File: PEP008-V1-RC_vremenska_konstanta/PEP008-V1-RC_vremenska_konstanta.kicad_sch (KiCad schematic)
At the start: 23 parts, among them J1 Screw_Terminal_01x02

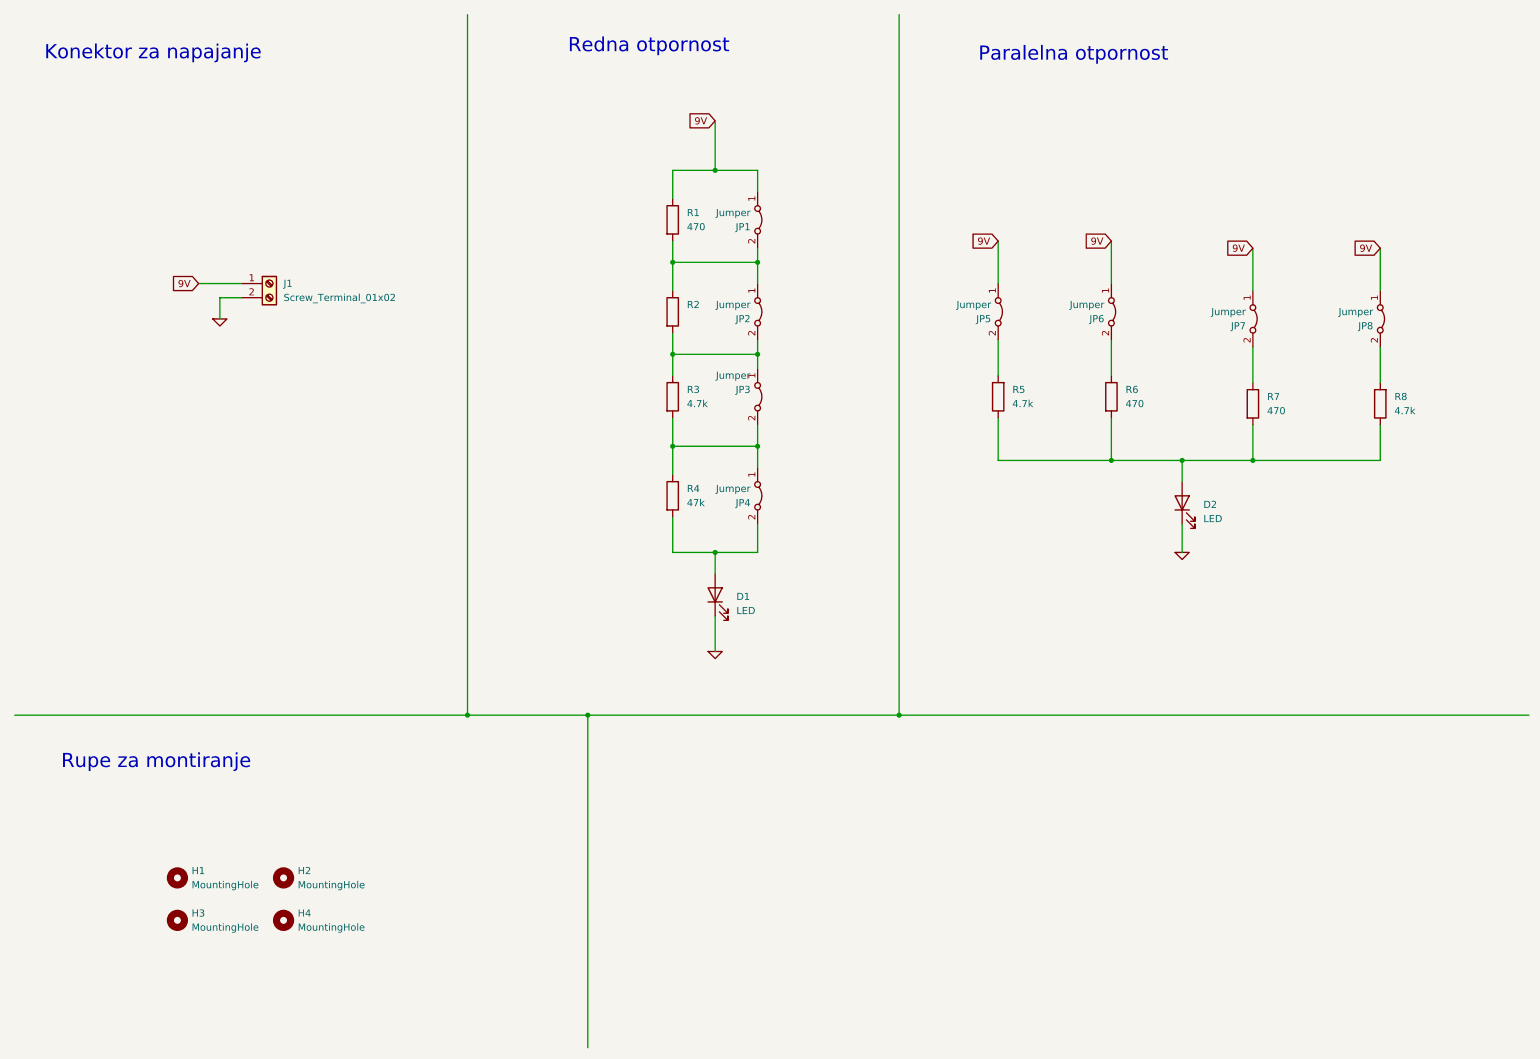
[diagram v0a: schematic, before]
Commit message: 3, 4, 8.
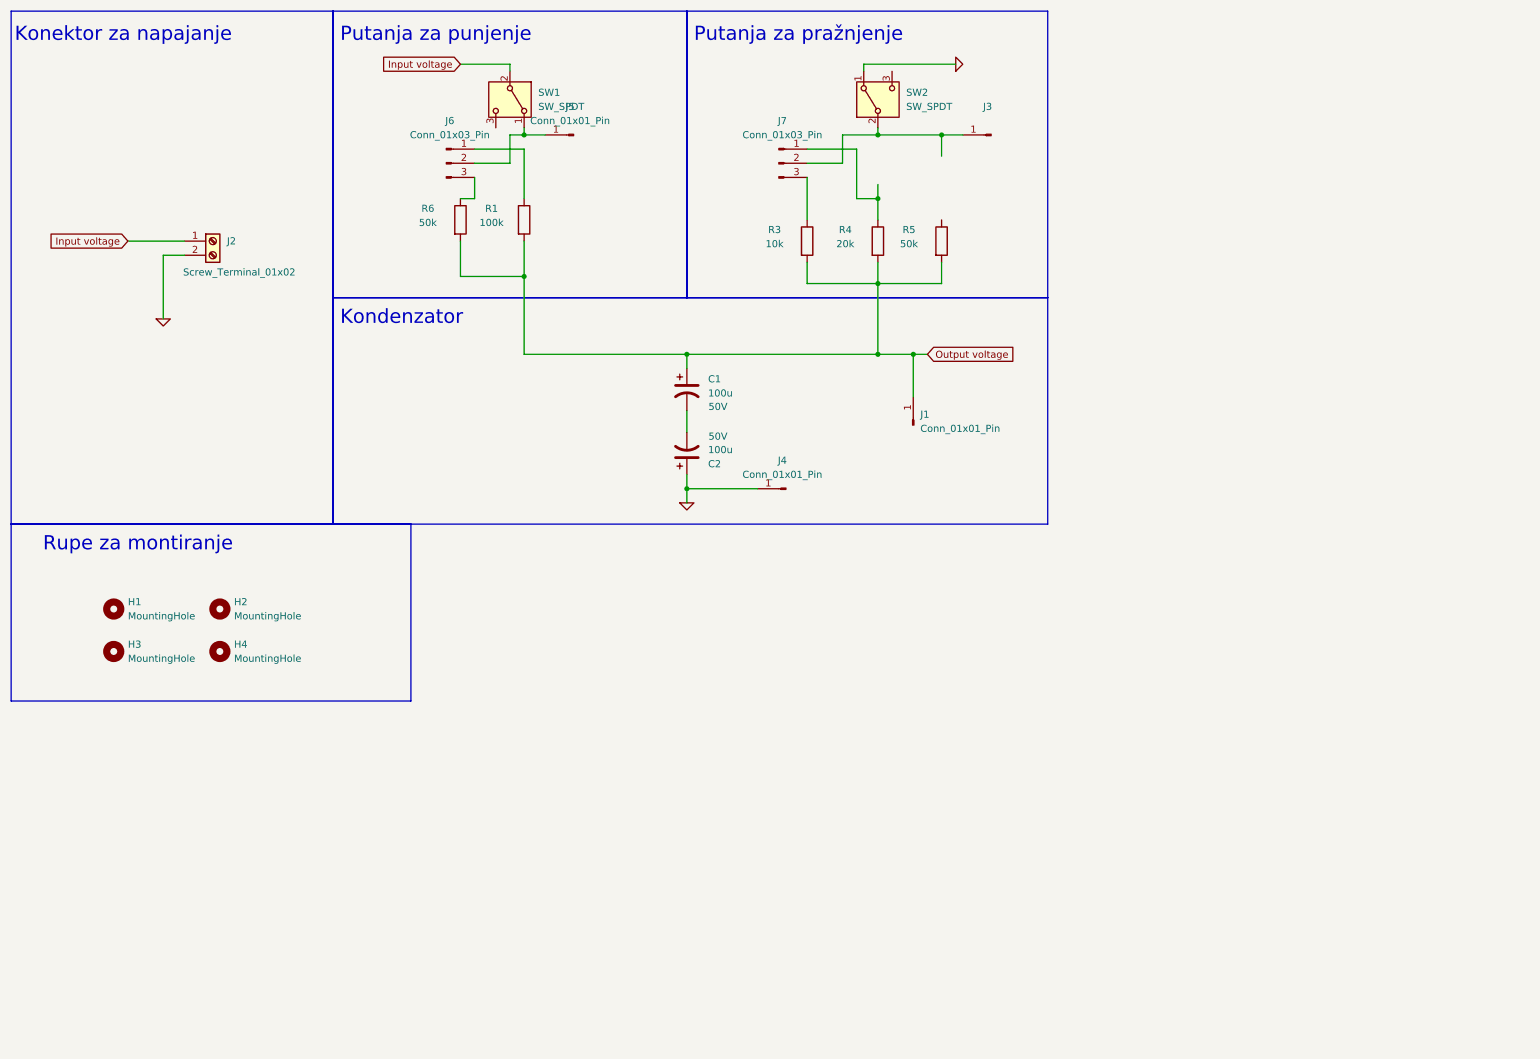
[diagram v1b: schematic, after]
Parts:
- removed D1, D2: LED, LED_SMD:LED_1206_3216Metric_Pad1.42x1.75mm_HandSolder, symbol Device:LED
- removed J1: Screw_Terminal_01x02, TerminalBlock_Phoenix:TerminalBlock_Phoenix_MKDS-1,5-2-5.08_1x02_P5.08mm_Horizontal, symbol Connector:Screw_Terminal_01x02
- removed JP1, JP2, JP3, JP4, JP5, JP6, JP7, JP8: Jumper, Connector_PinHeader_2.54mm:PinHeader_1x02_P2.54mm_Vertical, symbol Jumper:Jumper_2_Bridged
- removed R2: ~, Resistor_SMD:R_1206_3216Metric_Pad1.30x1.75mm_HandSolder, symbol Device:R
- removed R7: 470, Resistor_SMD:R_1206_3216Metric_Pad1.30x1.75mm_HandSolder, symbol Device:R
- removed R8: 4.7k, Resistor_SMD:R_1206_3216Metric_Pad1.30x1.75mm_HandSolder, symbol Device:R
- added C1, C2: 100u, Capacitor_THT:CP_Radial_D8.0mm_P3.50mm, symbol Device:C_Polarized_US
- added J1, J3, J4, J5: Conn_01x01_Pin, Connector_PinHeader_2.54mm:PinHeader_1x01_P2.54mm_Vertical, symbol Connector:Conn_01x01_Pin
- added J2: Screw_Terminal_01x02, TerminalBlock_Phoenix:TerminalBlock_Phoenix_MKDS-1,5-2-5.08_1x02_P5.08mm_Horizontal, symbol Connector:Screw_Terminal_01x02
- added J6, J7: Conn_01x03_Pin, symbol Connector:Conn_01x03_Pin
- added SW1, SW2: SW_SPDT, Button_Switch_THT:SW_E-Switch_EG1224_SPDT_Angled, symbol Switch:SW_SPDT
- R1: value 470 -> 100k
- R3: value 4.7k -> 10k
- R4: value 47k -> 20k
- R5: value 4.7k -> 50k
- R6: value 470 -> 50k
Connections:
- net 0: now also C2.1, J2.2 (Pin_2), J4.1 (Pin_1), SW2.1 (A)
- net at R3.1: now also J7.3 (Pin_3)
- net at R4.1: now also J7.1 (Pin_1); no longer R3.2
- net Output voltage: now reaches R4.2
- net Output voltage: now also R1.2, R3.2, R5.2, R6.2, C1.1, J1.1 (Pin_1)
- net at R5.1: no longer R6.2
- net at R6.1: now also J6.3 (Pin_3)
- net 9V: no longer names the net of R1.1
- net 9V: now also J6.1 (Pin_1)
- new net: J3.1 (Pin_1), J7.2 (Pin_2), SW2.2 (B)
- new net: J5.1 (Pin_1), J6.2 (Pin_2), SW1.1 (A)
- new net: C1.2, C2.2
- new net Input voltage: J2.1 (Pin_1), SW1.2 (B)
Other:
- note added: "Kondenzator"
- note added: "Putanja za pražnjenje"
- note added: "Putanja za punjenje"
- note removed: "Paralelna otpornost"
- note removed: "Redna otpornost"
- title: Redna i paralelna otpornost -> Punjenje i praznjenje kondenzatora
- moved on the sheet: H1, H2, H3, H4
